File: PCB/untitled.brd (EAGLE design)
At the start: 160 x 100 mm, 31 parts

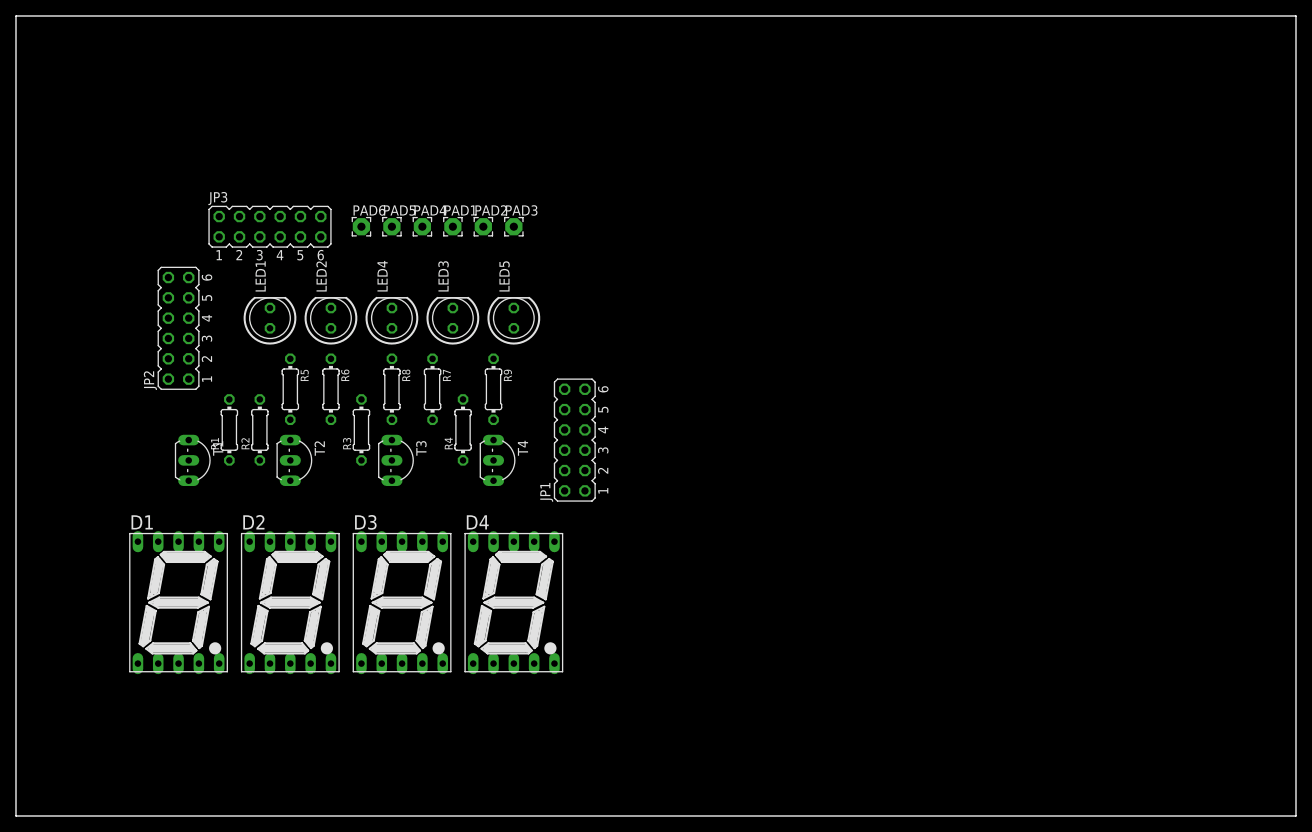
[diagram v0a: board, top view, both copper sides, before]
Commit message: Add files via upload
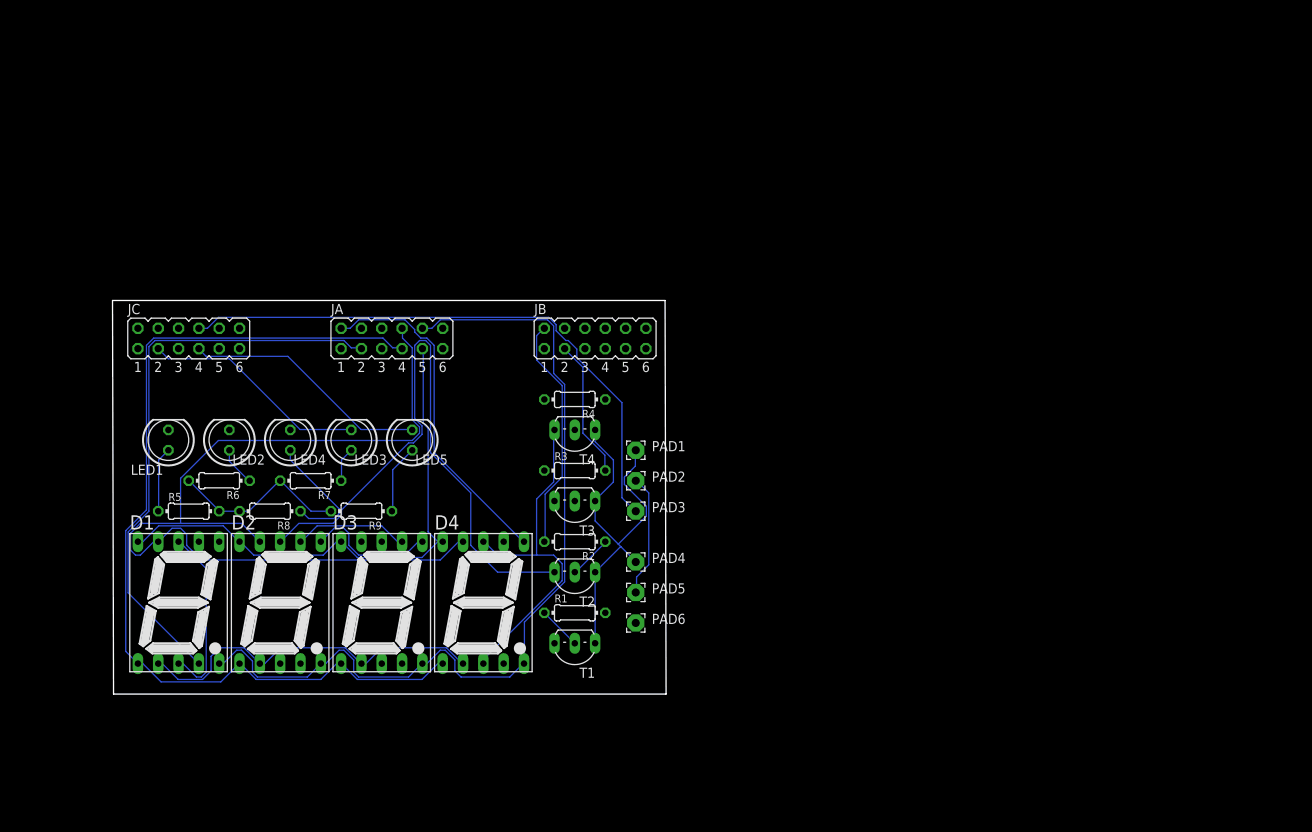
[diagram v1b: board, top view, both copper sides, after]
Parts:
- removed JP1, JP2, JP3: (no value), jumper:JP6Q
- added JA, JB, JC: (no value), jumper:JP6Q
- moved PAD6 60.2 mm to (77.5, 24.1), turned to 90 degrees
- moved PAD5 54.9 mm to (77.5, 27.9), turned to 90 degrees
- moved T1 52.8 mm to (69.8, 20.3), turned to 180 degrees
- moved PAD4 49.7 mm to (77.5, 31.8), turned to 90 degrees
- moved R1 48.9 mm to (69.8, 25.4), turned to 0 degrees
- moved R2 41.8 mm to (69.8, 34.3), turned to 180 degrees
- moved PAD3 38.7 mm to (77.5, 38.1), turned to 90 degrees
- moved T2 37.5 mm to (69.8, 29.2), turned to 180 degrees
- moved PAD2 37.0 mm to (77.5, 41.9), turned to 90 degrees
- moved PAD1 36.1 mm to (77.5, 45.7), turned to 90 degrees
- moved R3 27.1 mm to (69.8, 43.2), turned to 0 degrees
- moved T3 22.5 mm to (69.8, 38.1), turned to 180 degrees
- moved R9 22.5 mm to (43.2, 38.1), turned to 180 degrees
- moved R8 21.6 mm to (31.8, 38.1), turned to 180 degrees
- moved R5 19.8 mm to (21.6, 38.1), turned to 0 degrees
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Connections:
- net N$1: now also JA.1; no longer JP1.1
- net N$2: now also JA.2; no longer JP1.2
- net N$23: now also JB.1; no longer JP2.1
- net N$24: now also JB.2; no longer JP2.2
- net N$25: now also JB.3; no longer JP2.3
- net N$26: now also JB.4; no longer JP2.4
- net N$27: now also JC.1; no longer JP3.1
- net N$28: now also JC.2; no longer JP3.2
- net N$29: now also JC.3; no longer JP3.3
- net N$3: now also JA.4; no longer JP1.4
- net N$30: now also JC.4; no longer JP3.4
- net N$31: now also JC.7; no longer JP3.7
- net N$32: now also JC.8; no longer JP3.8
- net N$33: now also JA.5; no longer JP1.5
- net N$34: now also JA.6; no longer JP1.6
- net N$4: now also JA.3; no longer JP1.3
- net N$5: now also JA.7; no longer JP1.7
- net N$6: now also JA.8; no longer JP1.8
- net N$7: now also JA.9; no longer JP1.9
- net N$8: now also JA.10; no longer JP1.10
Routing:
- net N$6: track 0.00 -> 147.9 mm
- net N$13: track 0.00 -> 124.8 mm
- net N$5: track 0.00 -> 117.6 mm
- net N$4: track 0.00 -> 112.3 mm
- net N$8: track 0.00 -> 111.0 mm
- net N$10: track 0.00 -> 91.9 mm
- net N$3: track 0.00 -> 89.0 mm
- net N$2: track 0.00 -> 86.9 mm
- net N$32: track 0.00 -> 73.2 mm
- net N$9: track 0.00 -> 71.5 mm
- net N$7: track 0.00 -> 67.7 mm
- net N$34: track 0.00 -> 67.7 mm
- net N$1: track 0.00 -> 67.1 mm
- net N$33: track 0.00 -> 63.8 mm
- net N$12: track 0.00 -> 44.2 mm
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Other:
- board size 160 x 100 mm -> 69.2 x 49.2 mm
- board text added: "+5V hall sensor"
- board text added: "GND"
- board text added: "GND hall sensor"
- board text added: "IN +5V"
- board text added: "OUT +3,3V"
- board text added: "distance [km]"
- board text added: "hall sensor digital"
- board text added: "kcal"
- board text added: "max speed"
- board text added: "speed [km/h]"
- board text added: "time"
